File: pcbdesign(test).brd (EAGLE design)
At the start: 58.1 x 68.6 mm, 7 parts

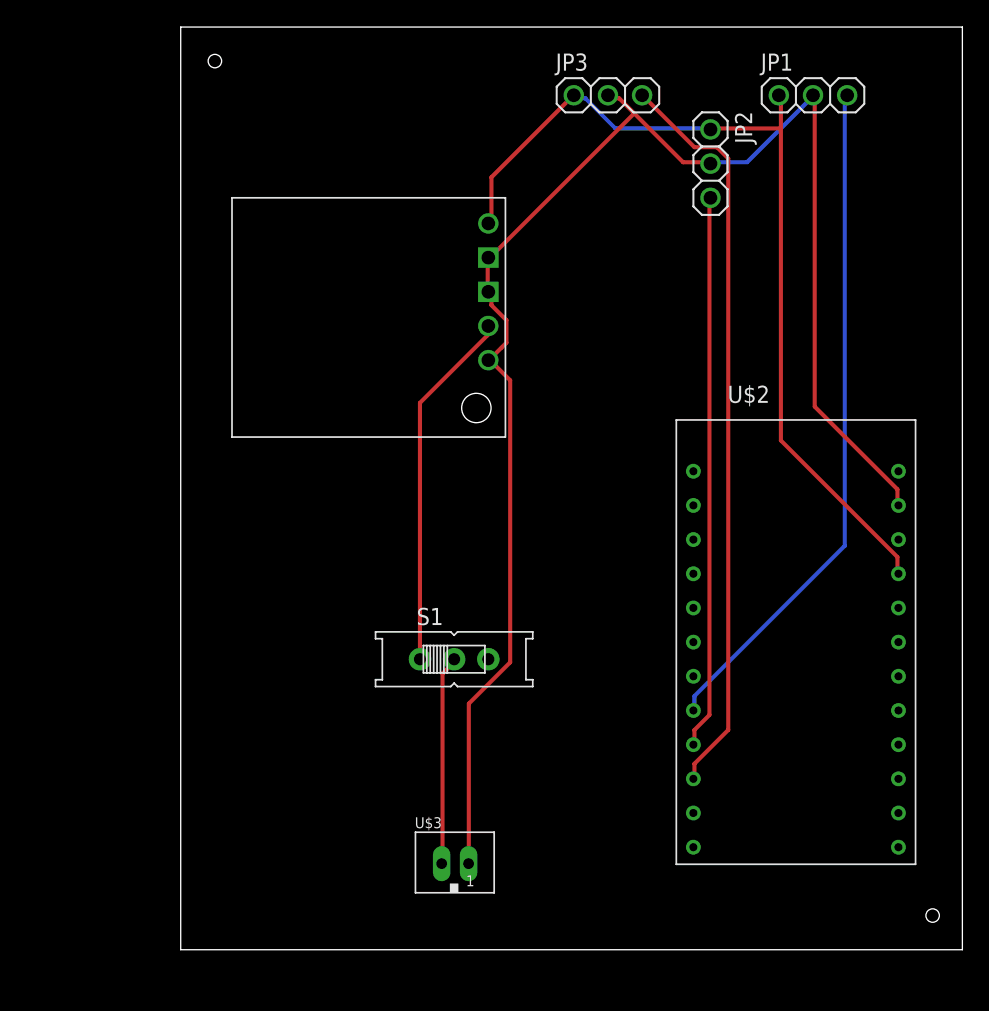
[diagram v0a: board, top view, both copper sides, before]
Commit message: Add files via upload
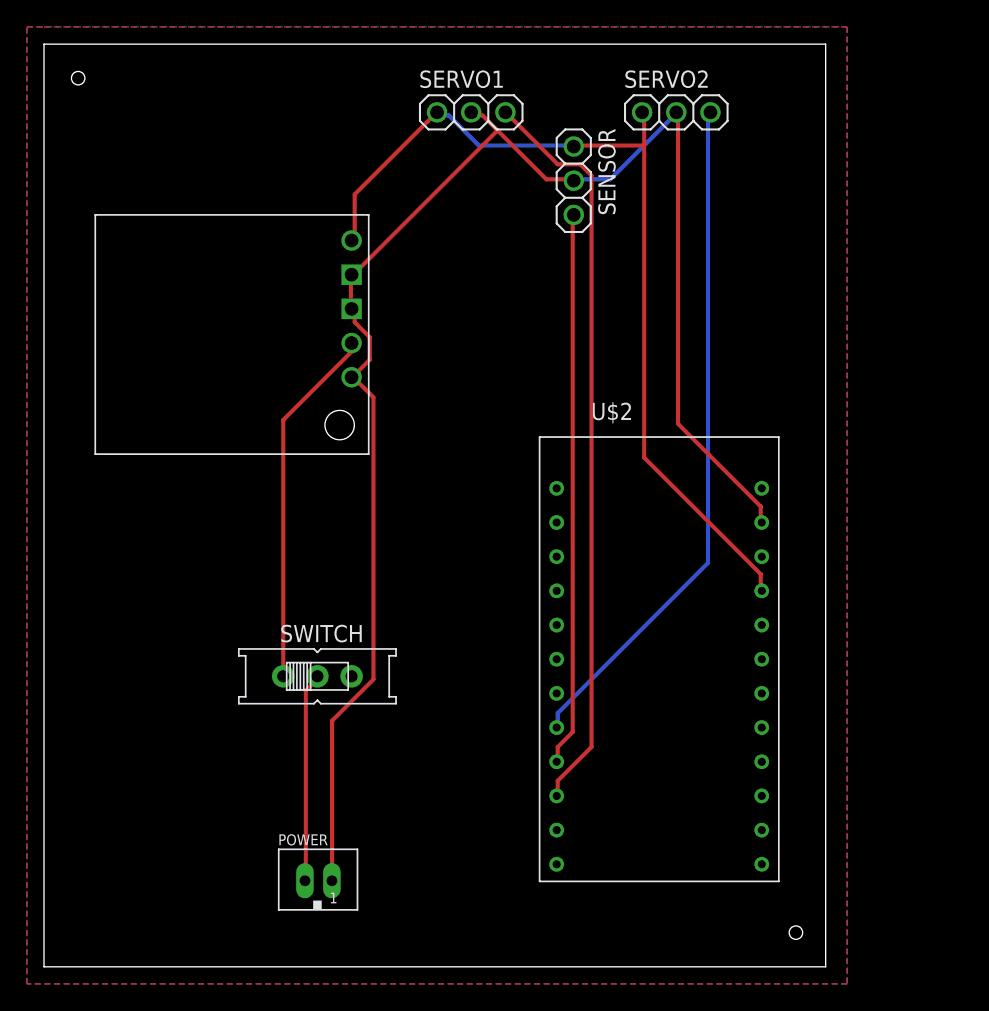
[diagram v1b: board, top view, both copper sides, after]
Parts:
- removed JP1, JP2, JP3: (no value), adafruit:1X03
- removed S1: (no value), adafruit:EG1218
- removed U$1: 5ASTEP-DOWNVOLTAGEREGULATOR, oddWorld:REG15D
- removed U$3: JST-PH_2-PIN_HEADER, SRG:JST_B2B-PH_HEADER
- added POWER: JST-PH_2-PIN_HEADER, SRG:JST_B2B-PH_HEADER
- added SENSOR, SERVO1, SERVO2: (no value), adafruit:1X03
- added SWITCH: (no value), adafruit:EG1218
- added V_REGULATOR: 5ASTEP-DOWNVOLTAGEREGULATOR, oddWorld:REG15D
- moved U$2 10.2 mm to (36.8, 6.35)
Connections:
- net 7.4V: now also POWER.P2, SWITCH.P; no longer S1.P, U$3.P2
- net GND: now also POWER.P1, SENSOR.2, SERVO1.2, SERVO2.2, V_REGULATOR.EN, V_REGULATOR.GND, V_REGULATOR.GND1; no longer JP1.2, JP2.2, JP3.2, U$1.EN, U$1.GND, U$1.GND1, U$3.P1
- net N$1: now also SERVO2.3; no longer JP1.3
- net N$2: now also SENSOR.3; no longer JP2.3
- net N$3: now also SERVO1.3; no longer JP3.3
- net N$4: now also SWITCH.O, V_REGULATOR.VIN; no longer S1.O, U$1.VIN
- net VCC: now also SENSOR.1, SERVO1.1, SERVO2.1, V_REGULATOR.VOUT; no longer JP1.1, JP2.1, JP3.1, U$1.VOUT
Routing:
- added copper zone on layer 1, net GND
- added copper zone on layer 16, net GND
